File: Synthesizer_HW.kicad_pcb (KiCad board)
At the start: 2 copper layers, 142.5 x 77.2 mm, 116 parts, among them J1 +5V_DC, J1&1 Selector, J2 USB_B_Micro, J3 EXT_REF_IN, J4 RF OUT1, J5 RF OUT2, Q1 BC857, Q2 BC847, Q3 BC847, Q4 IRLML5203, Q5 IRLML5203, U1 USBLC6-2, U2 SN74LVC1G3157, U3 STM32F042F6Px, U4 MAX2871, U5 GVA-63+, U6 XX1002-QH, U7 LT3042xMSE, U8 LP5907MFX-3.3, X1 TXETALSANF-10MHz

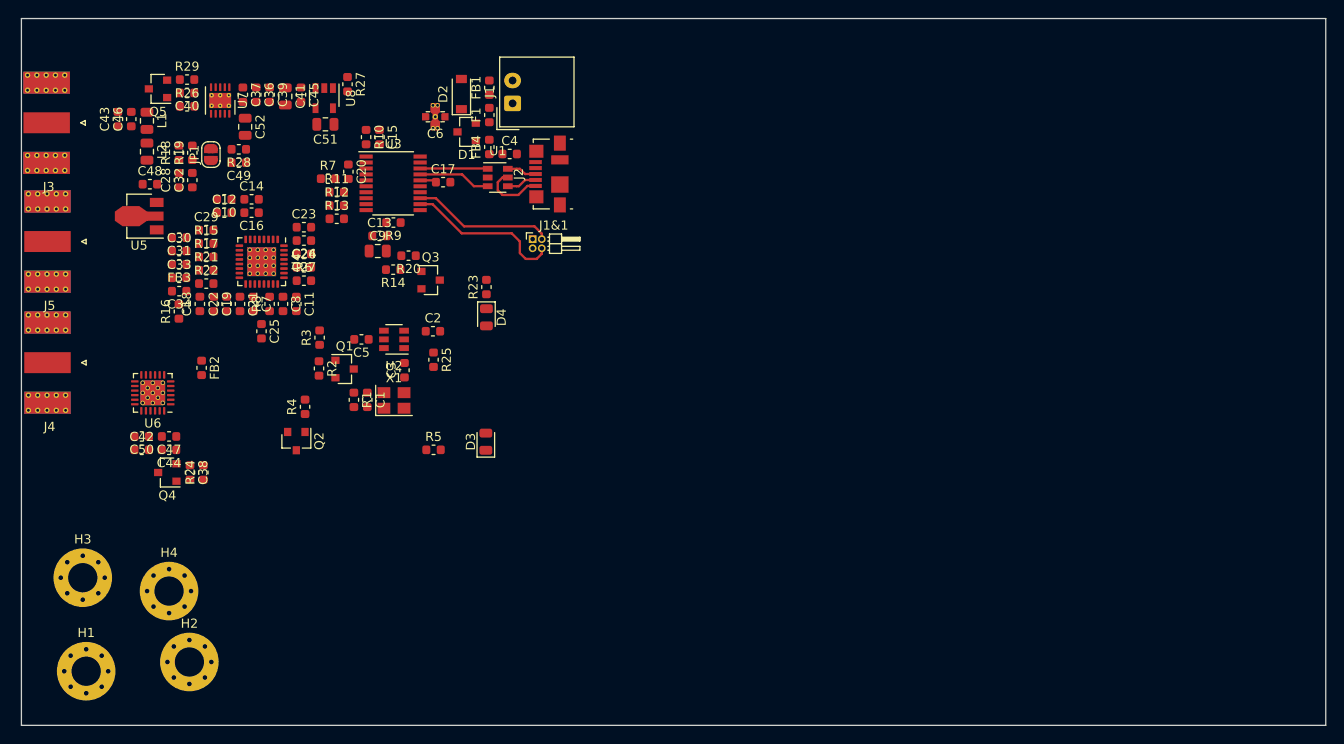
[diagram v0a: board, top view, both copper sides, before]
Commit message: board WIP, now editing silkscreen
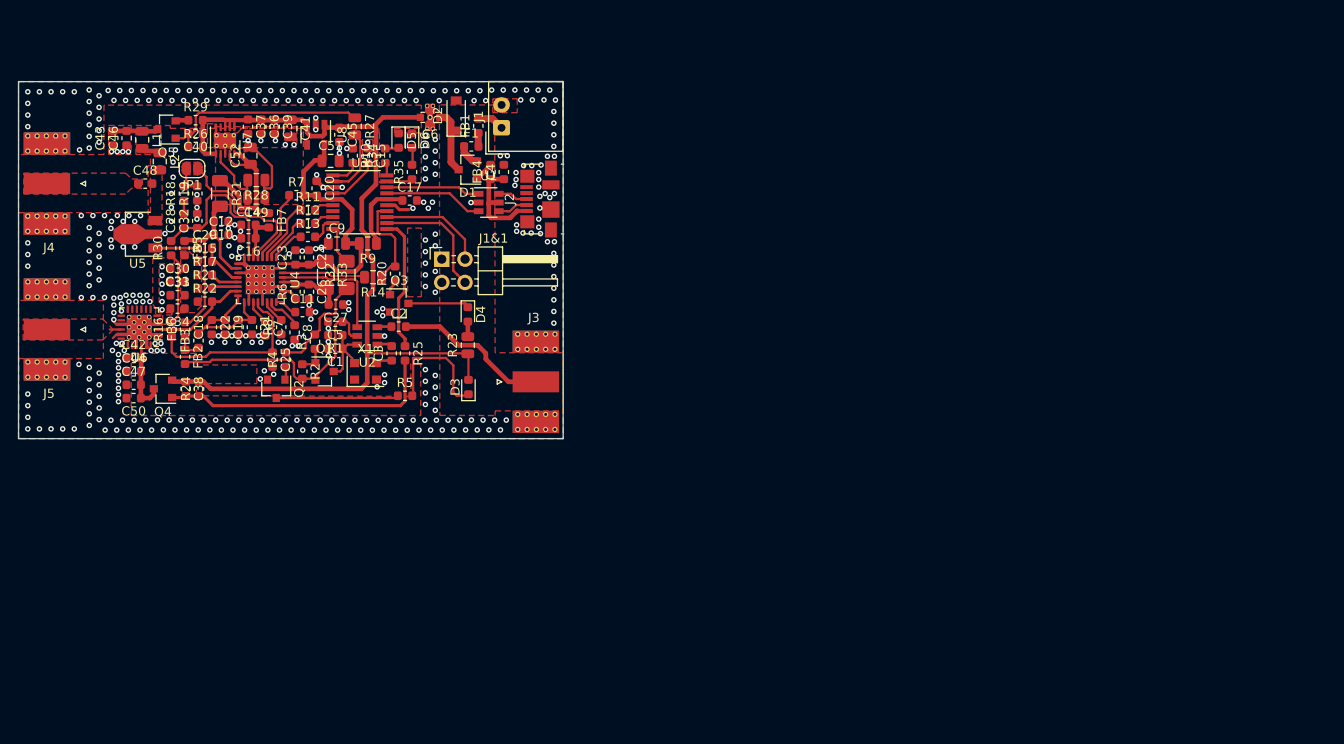
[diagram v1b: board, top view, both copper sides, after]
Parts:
- removed C13: 100n, Capacitor_SMD:C_0603_1608Metric
- removed H1, H2, H3, H4: MountingHole_Pad, MountingHole:MountingHole_3.2mm_M3_Pad_Via
- added D5: Status1, LED_SMD:LED_0603_1608Metric, F.Cu at (140.5, 51.9)
- added D6: Status2, LED_SMD:LED_0603_1608Metric, F.Cu at (142.0, 51.9)
- added FB5: BLM18PG471, Inductor_SMD:L_0603_1608Metric, F.Cu at (117.1, 63.7)
- added FB6: BLM18PG471, Inductor_SMD:L_0603_1608Metric, F.Cu at (117.2, 72.6)
- added FB7: BLM18PG471, Inductor_SMD:L_0603_1608Metric, F.Cu at (126.3, 60.6)
- added R30: 0R, Resistor_SMD:R_0603_1608Metric, F.Cu at (115.7, 63.7)
- added R31: 0R, Resistor_SMD:R_1206_3216Metric, F.Cu at (121.0, 57.7)
- added R32: 0R, Resistor_SMD:R_1206_3216Metric_Pad1.42x1.75mm_HandSolder, F.Cu at (134.8, 66.6)
- added R33: 0R, Resistor_SMD:R_1206_3216Metric_Pad1.42x1.75mm_HandSolder, F.Cu at (132.6, 66.6)
- added R34: 1k, Resistor_SMD:R_0603_1608Metric, F.Cu at (139.1, 53.6)
- added R35: 1k, Resistor_SMD:R_0603_1608Metric, F.Cu at (142.0, 55.4)
- C49: footprint Capacitor_SMD:C_0603_1608Metric -> Capacitor_SMD:C_0805_2012Metric
- D3, D4: footprint LED_SMD:LED_0805_2012Metric -> LED_SMD:LED_0603_1608Metric
- J1&1: footprint Connector_PinHeader_1.00mm:PinHeader_2x02_P1.00mm_Horizontal -> Connector_PinHeader_2.54mm:PinHeader_2x02_P2.54mm_Horizontal
- R14, R23, R27, R28, R9: footprint Resistor_SMD:R_0603_1608Metric -> Resistor_SMD:R_0805_2012Metric
- X1: footprint Crystal:Crystal_SMD_Abracon_ABM8G-4Pin_3.2x2.5mm -> KLALIB_Crystal:Crystal_SMD_4Pin_3.2x2.5mm
- moved J3 57.4 mm to (153.8, 78.3), turned to 180 degrees
- moved J4 19.6 mm to (103.8, 56.6)
- moved J1&1 10.2 mm to (145.2, 64.9)
- moved C42 10.1 mm to (111.6, 75.7)
- moved J5 9.61 mm to (103.8, 72.6)
- moved C44 9.40 mm to (111.6, 77.2), turned to 0 degrees
- moved C38 9.16 mm to (117.3, 79.1)
- moved Q4 9.16 mm to (114.8, 79.1)
- moved R24 9.16 mm to (118.7, 79.1)
- moved FB3 8.58 mm to (118.7, 73.8), turned to 90 degrees
- moved R1 7.35 mm to (133.6, 73.2), turned to 180 degrees
- moved U6 7.33 mm to (112.2, 72.3)
- moved C47 6.84 mm to (111.6, 78.6), turned to 0 degrees
- moved R5 6.68 mm to (141.2, 79.8)
- moved R23 6.67 mm to (148.1, 74.3)
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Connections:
- C10 pad 2: VDDA -> Net-(C10-Pad2)
- C12 pad 1: VDDA -> Net-(C10-Pad2)
- C14 pad 2: VDDA -> Net-(C14-Pad2)
- C16 pad 1: VDDA -> Net-(C14-Pad2)
- C26 pad 1: VDD -> /VDD1
- C27 pad 2: VDD -> /VDD1
- C30 pad 2: VDDA -> Net-(C30-Pad2)
- C31 pad 1: VDDA -> Net-(C30-Pad2)
- C33 pad 2: VDDA -> Net-(C30-Pad2)
- C34 pad 1: VDDA -> Net-(C30-Pad2)
- D4 pad 2: +5V -> Net-(D4-Pad2)
- FB2 pad 1: VDDA -> Net-(FB2-Pad1)
- FB3 pad 1: VDDA -> Net-(FB2-Pad1)
- J1 pad 1: GND -> Net-(FB1-Pad2)
- J1 pad 2: Net-(FB1-Pad2) -> GND
- Q3 pad 3: Net-(Q3-Pad3) -> Net-(D4-Pad1)
- R15 pad 1: VDDA -> Net-(C30-Pad2)
- R16 pad 2: Net-(C28-Pad1) -> Net-(R16-Pad2)
- R17 pad 1: VDDA -> Net-(C30-Pad2)
- R21 pad 1: VDDA -> Net-(C30-Pad2)
- R22 pad 1: VDDA -> Net-(C30-Pad2)
- R23 pad 1: Net-(D4-Pad1) -> +5V
- R23 pad 2: Net-(Q3-Pad3) -> Net-(D4-Pad2)
- R6 pad 2: VDD -> /VDD1
- U3 pad 10: /INT_REF -> Net-(R32-Pad2)
- U3 pad 19: (no net) -> Net-(R35-Pad1)
- U3 pad 20: (no net) -> Net-(R34-Pad1)
- U4 pad 10: VDDA -> Net-(C10-Pad2)
- U4 pad 28: VDD -> /VDD1
- U4 pad 6: VDDA -> Net-(C14-Pad2)
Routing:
- net +5V: track 0.00 -> 99.1 mm
- net GND: track 0.00 -> 52.6 mm, vias 0 -> 393
- net VDD: track 0.00 -> 30.6 mm
- net Net-(C38-Pad2): track 0.00 -> 30.6 mm
- net Net-(C5-Pad1): track 0.00 -> 26.4 mm
- net Net-(C40-Pad2): track 0.00 -> 23.1 mm
- net Net-(C10-Pad2): track 0.00 -> 21.9 mm
- net Net-(C25-Pad1): track 0.00 -> 19.9 mm
- net VDDA: track 0.00 -> 18.2 mm
- net Net-(C28-Pad1): track 0.00 -> 18.0 mm
- net Net-(C2-Pad2): track 0.00 -> 17.2 mm
- net Net-(JP1-Pad1): track 0.00 -> 17.1 mm
- net /DOUBLER_EN: track 0.00 -> 14.8 mm
- net Net-(C18-Pad2): track 0.00 -> 14.2 mm
- net Net-(D3-Pad1): track 0.00 -> 13.7 mm
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- added copper zone on B.Cu, net GND
- added copper zone on F.Cu, net GND
- added copper zone on F.Cu, net Net-(C30-Pad2)
- added copper zone on F.Cu, net Net-(C48-Pad1)
- added copper zone on F.Cu, net Net-(C48-Pad2)
- added copper zone on F.Cu, net Net-(J5-Pad1)
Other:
- board size 142.5 x 77.2 mm -> 59.5 x 39 mm
- net class Default: trace_width 0.25 -> 0.254; via_dia 0.8 -> 0.6; via_drill 0.4 -> 0.3
- rule trace_min: 0.1524 -> 0
- rule via_min_size: 0.4 -> 0.6
